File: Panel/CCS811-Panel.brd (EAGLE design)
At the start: 54.4 x 54.4 mm, 162 parts, among them U1 CCS811PRODUCTION, U2 CCS811PRODUCTION, U3 CCS811PRODUCTION, U4 CCS811PRODUCTION, U5 CCS811PRODUCTION, U6 CCS811PRODUCTION, U7 CCS811PRODUCTION, U8 CCS811PRODUCTION, U9 CCS811PRODUCTION

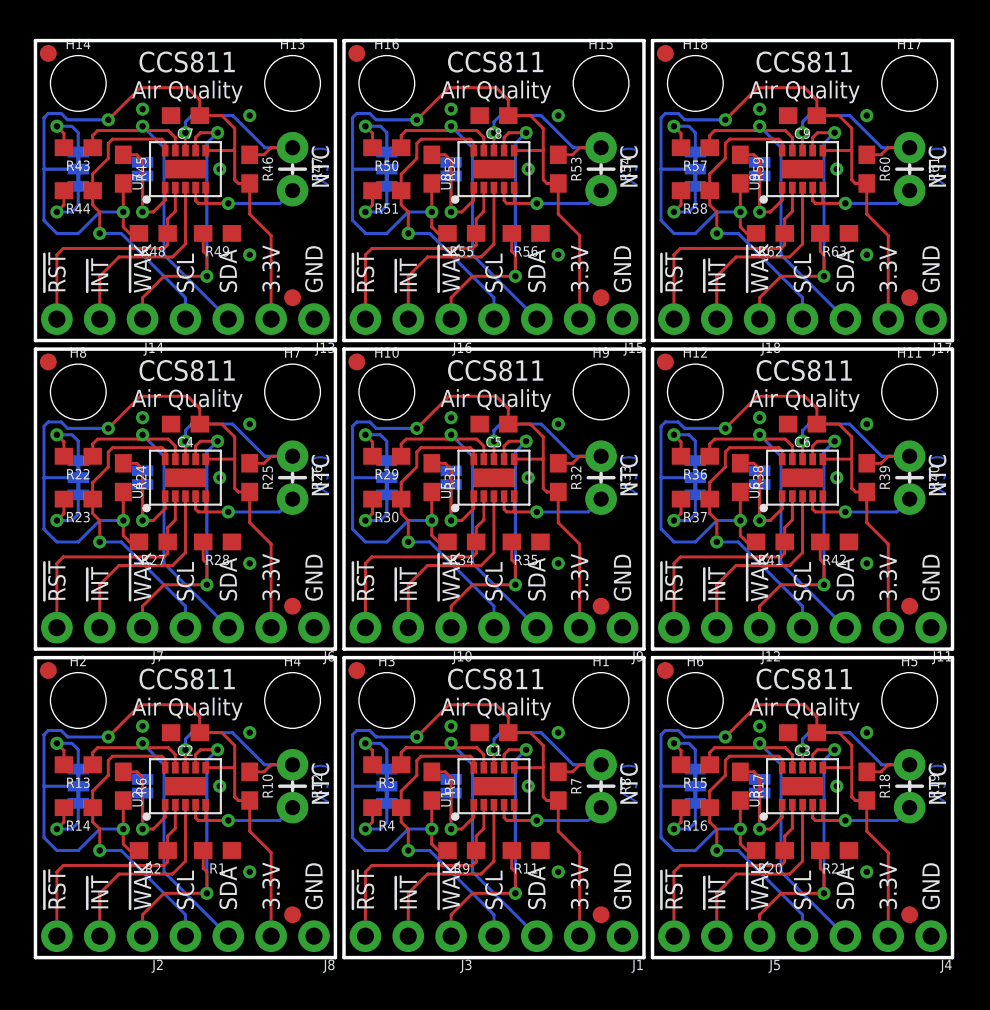
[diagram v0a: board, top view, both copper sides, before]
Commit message: Reviewed and fixed Panel
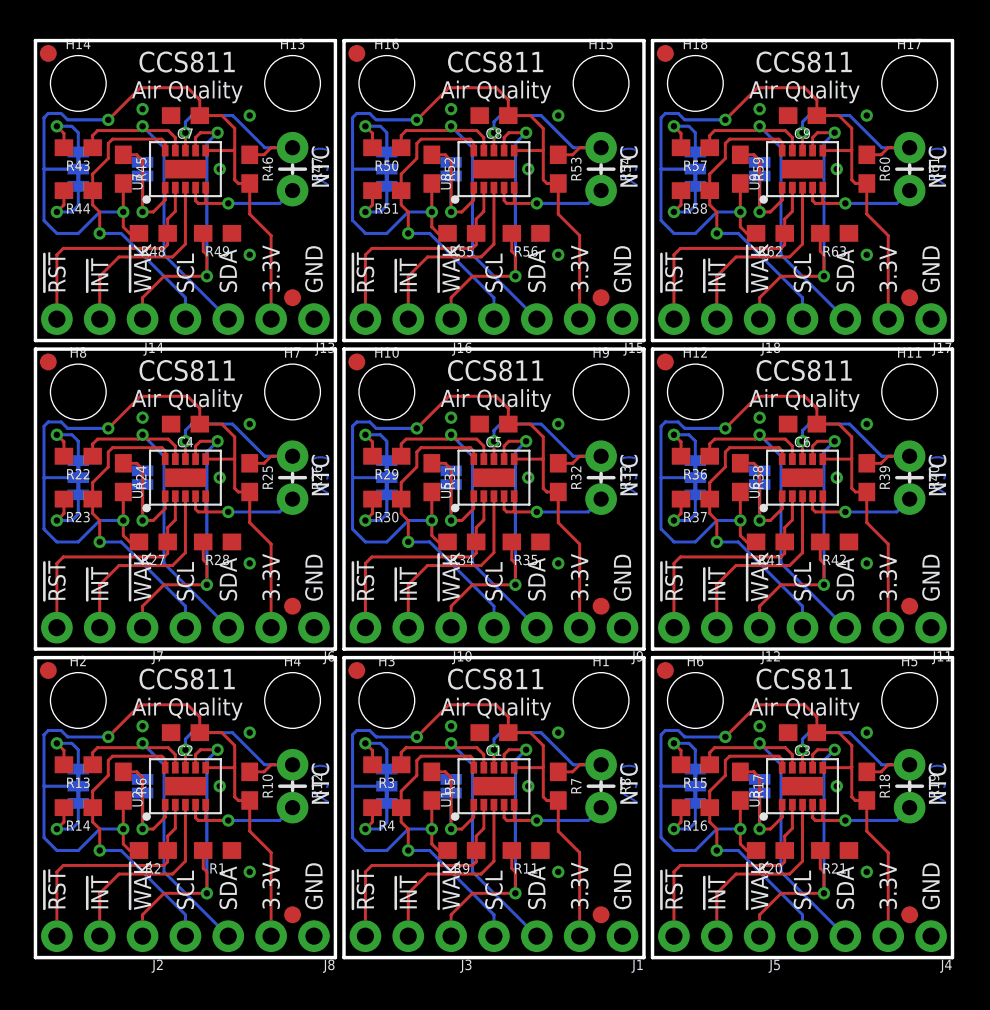
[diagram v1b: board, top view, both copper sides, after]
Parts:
- added LOGO1, LOGO2, LOGO3, LOGO4, LOGO5, LOGO6, LOGO7, LOGO8, LOGO9: OSHW-LOGOS, SparkFun-Aesthetics:OSHW-LOGO-S
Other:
- board text added: "ADDR"
- board text added: "I2C PU"
- board text removed: "JP1"
- board text removed: "JP2"
